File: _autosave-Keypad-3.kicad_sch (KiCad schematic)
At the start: 20 parts, among them SW1 SW_Push, U1 ATmega32U4-A, Y1 16MHz

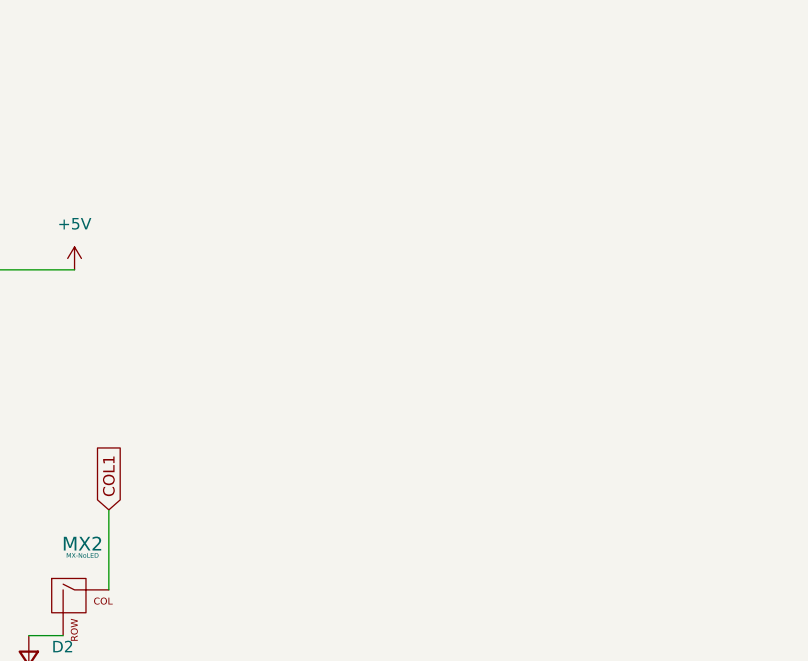
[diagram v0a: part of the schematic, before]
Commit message: Finished first board design
route is very messy, will fix soon.
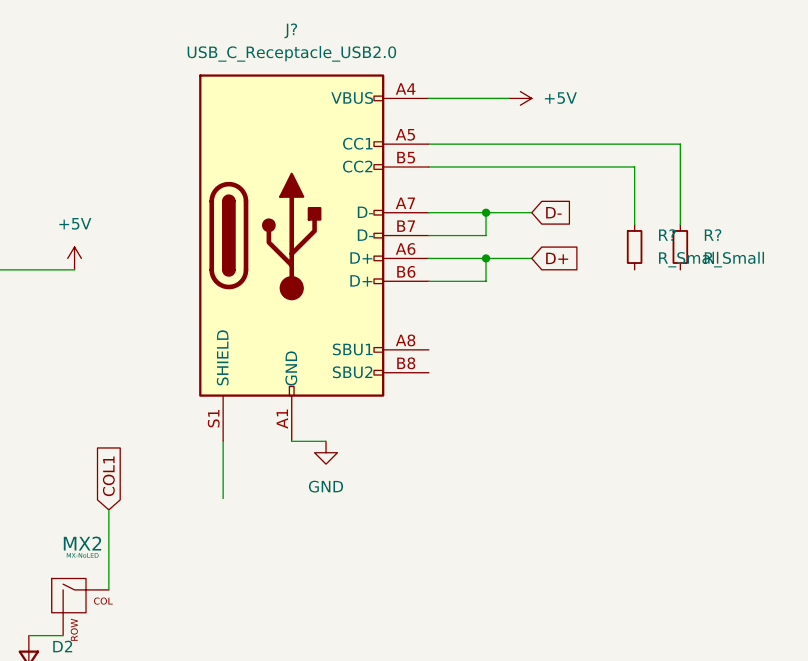
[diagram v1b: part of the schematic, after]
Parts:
- added J?: USB_C_Receptacle_USB2.0, symbol Connector:USB_C_Receptacle_USB2.0
- added R? (x2): R_Small, symbol Device:R_Small
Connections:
- net +5V: now also J?.A4 (VBUS), J?.A9 (VBUS), J?.B4 (VBUS), J?.B9 (VBUS)
- net D+: now also J?.A6 (D+), J?.B6 (D+)
- net D-: now also J?.A7 (D-), J?.B7 (D-)
- net GND: now also J?.A1 (GND), J?.A12 (GND), J?.B1 (GND), J?.B12 (GND)
- new net: J?.B5 (CC2), R?.1
- new net: J?.A5 (CC1), R?.1
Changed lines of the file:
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@@
 (kicad_sch (version 20211123) (generator eeschema)
   (paper "A4")
+  (junction (at 241.3 35.56) (diameter 0) (color 0 0 0 0)
+  )
   (junction (at 114.3 35.56) (diameter 0) (color 0 0 0 0)
   )
@@
   (junction (at 74.93 54.61) (diameter 0) (color 0 0 0 0)
   )
+  (junction (at 241.3 40.64) (diameter 0) (color 0 0 0 0)
+  )
   (junction (at 60.96 111.76) (diameter 0) (color 0 0 0 0)
   )
@@
     (stroke (width 0) (type default) (color 0 0 0 0))
   )
+  (wire (pts (xy 234.95 43.18) (xy 241.3 43.18))
+    (stroke (width 0) (type default) (color 0 0 0 0))
+  )
   (wire (pts (xy 96.52 43.18) (xy 99.06 43.18))
     (stroke (width 0) (type default) (color 0 0 0 0))
   )
+  (wire (pts (xy 212.09 60.96) (xy 212.09 67.31))
+    (stroke (width 0) (type default) (color 0 0 0 0))
+  )
   (wire (pts (xy 172.72 41.91) (xy 181.61 41.91))
     (stroke (width 0) (type default) (color 0 0 0 0))
@@
     (stroke (width 0) (type default) (color 0 0 0 0))
   )
+  (wire (pts (xy 234.95 30.48) (xy 257.81 30.48))
+    (stroke (width 0) (type default) (color 0 0 0 0))
+  )
+  (wire (pts (xy 234.95 22.86) (xy 243.84 22.86))
+    (stroke (width 0) (type default) (color 0 0 0 0))
+  )
   (wire (pts (xy 86.36 48.26) (xy 80.01 48.26))
     (stroke (width 0) (type default) (color 0 0 0 0))
@@
     (stroke (width 0) (type default) (color 0 0 0 0))
   )
+  (wire (pts (xy 234.95 35.56) (xy 241.3 35.56))
+    (stroke (width 0) (type default) (color 0 0 0 0))
+  )
+  (wire (pts (xy 257.81 30.48) (xy 257.81 36.83))
+    (stroke (width 0) (type default) (color 0 0 0 0))
+  )
   (wire (pts (xy 69.85 71.12) (xy 74.93 71.12))
     (stroke (width 0) (type default) (color 0 0 0 0))
@@
     (stroke (width 0) (type default) (color 0 0 0 0))
   )
+  (wire (pts (xy 241.3 40.64) (xy 246.38 40.64))
+    (stroke (width 0) (type default) (color 0 0 0 0))
+  )
   (wire (pts (xy 73.66 76.2) (xy 99.06 76.2))
     (stroke (width 0) (type default) (color 0 0 0 0))
   )
+  (wire (pts (xy 234.95 38.1) (xy 241.3 38.1))
+    (stroke (width 0) (type default) (color 0 0 0 0))
+  )
   (wire (pts (xy 93.98 43.18) (xy 96.52 43.18))
     (stroke (width 0) (type default) (color 0 0 0 0))
@@
     (stroke (width 0) (type default) (color 0 0 0 0))
   )
+  (wire (pts (xy 262.89 27.94) (xy 262.89 36.83))
+    (stroke (width 0) (type default) (color 0 0 0 0))
+  )
   (wire (pts (xy 83.82 50.8) (xy 83.82 55.88))
     (stroke (width 0) (type default) (color 0 0 0 0))
@@
     (stroke (width 0) (type default) (color 0 0 0 0))
   )
+  (wire (pts (xy 241.3 35.56) (xy 246.38 35.56))
+    (stroke (width 0) (type default) (color 0 0 0 0))
+  )
   (wire (pts (xy 86.36 53.34) (xy 99.06 53.34))
     (stroke (width 0) (type default) (color 0 0 0 0))
@@
     (stroke (width 0) (type default) (color 0 0 0 0))
   )
+  (wire (pts (xy 241.3 35.56) (xy 241.3 38.1))
+    (stroke (width 0) (type default) (color 0 0 0 0))
+  )
   (wire (pts (xy 66.04 106.68) (xy 76.2 106.68))
     (stroke (width 0) (type default) (color 0 0 0 0))
@@
     (stroke (width 0) (type default) (color 0 0 0 0))
   )
+  (wire (pts (xy 219.71 60.96) (xy 223.52 60.96))
+    (stroke (width 0) (type default) (color 0 0 0 0))
+  )
+  (wire (pts (xy 234.95 27.94) (xy 262.89 27.94))
+    (stroke (width 0) (type default) (color 0 0 0 0))
+  )
   (wire (pts (xy 45.72 111.76) (xy 55.88 111.76))
     (stroke (width 0) (type default) (color 0 0 0 0))
@@
     (stroke (width 0) (type default) (color 0 0 0 0))
   )
+  (wire (pts (xy 241.3 40.64) (xy 241.3 43.18))
+    (stroke (width 0) (type default) (color 0 0 0 0))
+  )
   (wire (pts (xy 55.88 111.76) (xy 60.96 111.76))
     (stroke (width 0) (type default) (color 0 0 0 0))
@@
   )
   (wire (pts (xy 74.93 54.61) (xy 74.93 58.42))
+    (stroke (width 0) (type default) (color 0 0 0 0))
+  )
+  (wire (pts (xy 234.95 40.64) (xy 241.3 40.64))
     (stroke (width 0) (type default) (color 0 0 0 0))
   )
@@
     )
   )
+  (global_label "D-" (shape input) (at 246.38 35.56 0) (fields_autoplaced)
+    (effects (font (size 1.27 1.27)) (justify left))
+    (property "Intersheet References" "${INTERSHEET_REFS}" (id 0) (at 251.6355 35.4806 0)
+      (effects (font (size 1.27 1.27)) (justify left) hide)
+    )
+  )
   (global_label "COL0" (shape input) (at 129.54 114.3 0) (fields_autoplaced)
     (effects (font (size 1.27 1.27)) (justify left))
@@
     )
   )
+  (global_label "D+" (shape input) (at 246.38 40.64 0) (fields_autoplaced)
+    (effects (font (size 1.27 1.27)) (justify left))
+    (property "Intersheet References" "${INTERSHEET_REFS}" (id 0) (at 251.6355 40.5606 0)
+      (effects (font (size 1.27 1.27)) (justify left) hide)
+    )
+  )
   (global_label "D+" (shape input) (at 69.85 68.58 180) (fields_autoplaced)
     (effects (font (size 1.27 1.27)) (justify right))
@@
     (pin "1")
     (pin "2")
+  )
+  (symbol (lib_id "power:+5V") (at 243.84 22.86 270) (unit 1)
+    (in_bom yes) (on_board yes) (fields_autoplaced)
+    (property "Reference" "#PWR?" (id 0) (at 240.03 22.86 0)
+      (effects (font (size 1.27 1.27)) hide)
+    )
+    (property "Value" "+5V" (id 1) (at 247.65 22.8599 90)
+      (effects (font (size 1.27 1.27)) (justify left))
+    )
+    (property "Footprint" "" (id 2) (at 243.84 22.86 0)
+      (effects (font (size 1.27 1.27)) hide)
+    )
+    (property "Datasheet" "" (id 3) (at 243.84 22.86 0)
+      (effects (font (size 1.27 1.27)) hide)
+    )
+    (pin "1")
   )
   (symbol (lib_id "power:+5V") (at 195.58 41.91 0) (unit 1)
@@
     (pin "2")
   )
+  (symbol (lib_id "Device:R_Small") (at 257.81 39.37 0) (unit 1)
+    (in_bom yes) (on_board yes) (fields_autoplaced)
+    (property "Reference" "R?" (id 0) (at 260.35 38.0999 0)
+      (effects (font (size 1.27 1.27)) (justify left))
+    )
+    (property "Value" "R_Small" (id 1) (at 260.35 40.6399 0)
+      (effects (font (size 1.27 1.27)) (justify left))
+    )
+    (property "Footprint" "" (id 2) (at 257.81 39.37 0)
+      (effects (font (size 1.27 1.27)) hide)
+    )
+    (property "Datasheet" "~" (id 3) (at 257.81 39.37 0)
+      (effects (font (size 1.27 1.27)) hide)
+    )
+    (pin "1")
+    (pin "2")
+  )
   (symbol (lib_id "power:GND") (at 73.66 85.09 0) (unit 1)
     (in_bom yes) (on_board yes) (fields_autoplaced)
@@
     (pin "2")
   )
+  (symbol (lib_id "Device:R_Small") (at 262.89 39.37 0) (unit 1)
+    (in_bom yes) (on_board yes) (fields_autoplaced)
+    (property "Reference" "R?" (id 0) (at 265.43 38.0999 0)
+      (effects (font (size 1.27 1.27)) (justify left))
+    )
+    (property "Value" "R_Small" (id 1) (at 265.43 40.6399 0)
+      (effects (font (size 1.27 1.27)) (justify left))
+    )
+    (property "Footprint" "" (id 2) (at 262.89 39.37 0)
+      (effects (font (size 1.27 1.27)) hide)
+    )
+    (property "Datasheet" "~" (id 3) (at 262.89 39.37 0)
+      (effects (font (size 1.27 1.27)) hide)
+    )
+    (pin "1")
+    (pin "2")
+  )
   (symbol (lib_id "Device:C_Small") (at 66.04 109.22 0) (unit 1)
     (in_bom yes) (on_board yes) (fields_autoplaced)
@@
     )
     (pin "1")
+  )
+  (symbol (lib_id "Connector:USB_C_Receptacle_USB2.0") (at 219.71 38.1 0) (unit 1)
+    (in_bom yes) (on_board yes) (fields_autoplaced)
+    (property "Reference" "J?" (id 0) (at 219.71 15.24 0))
+    (property "Value" "USB_C_Receptacle_USB2.0" (id 1) (at 219.71 17.78 0))
+    (property "Footprint" "" (id 2) (at 223.52 38.1 0)
+      (effects (font (size 1.27 1.27)) hide)
+    )
+    (property "Datasheet" "https://www.usb.org/sites/default/files/documents/usb_type-c.zip" (id 3) (at 223.52 38.1 0)
+      (effects (font (size 1.27 1.27)) hide)
+    )
+    (pin "A1")
+    (pin "A12")
+    (pin "A4")
+    (pin "A5")
+    (pin "A6")
+    (pin "A7")
+    (pin "A8")
+    (pin "A9")
+    (pin "B1")
+    (pin "B12")
+    (pin "B4")
+    (pin "B5")
+    (pin "B6")
+    (pin "B7")
+    (pin "B8")
+    (pin "B9")
+    (pin "S1")
   )
   (symbol (lib_id "Device:Crystal_GND24_Small") (at 86.36 50.8 270) (unit 1)
@@
     (pin "1")
   )
+  (symbol (lib_id "power:GND") (at 223.52 60.96 0) (unit 1)
+    (in_bom yes) (on_board yes) (fields_autoplaced)
+    (property "Reference" "#PWR?" (id 0) (at 223.52 67.31 0)
+      (effects (font (size 1.27 1.27)) hide)
+    )
+    (property "Value" "GND" (id 1) (at 223.52 66.04 0))
+    (property "Footprint" "" (id 2) (at 223.52 60.96 0)
+      (effects (font (size 1.27 1.27)) hide)
+    )
+    (property "Datasheet" "" (id 3) (at 223.52 60.96 0)
+      (effects (font (size 1.27 1.27)) hide)
+    )
+    (pin "1")
+  )
   (sheet_instances
     (path "/" (page "1"))
@@
       (reference "#PWR0113") (unit 1) (value "VCC") (footprint "")
     )
+    (path "/3c27b9f9-2ba8-4150-8cd7-fc6b702be7b9"
+      (reference "#PWR?") (unit 1) (value "+5V") (footprint "")
+    )
+    (path "/ff0f6824-7994-4850-9e6c-74e9b0f18f76"
+      (reference "#PWR?") (unit 1) (value "GND") (footprint "")
+    )
     (path "/ad0e28b6-1443-4065-afe7-dc2a56df346b"
       (reference "C1") (unit 1) (value "22pf") (footprint "Capacitor_SMD:C_0805_2012Metric")
@@
       (reference "F1") (unit 1) (value "500mA") (footprint "Fuse:Fuse_1206_3216Metric")
     )
+    (path "/dcf57bfd-08d4-4b5b-9245-8eb742026298"
+      (reference "J?") (unit 1) (value "USB_C_Receptacle_USB2.0") (footprint "")
+    )
     (path "/728e0df7-77d3-4862-b864-13cb45a6d3ad"
       (reference "MX1") (unit 1) (value "MX-NoLED") (footprint "MX_Alps_Hybrid:MX-1U-NoLED")
@@
       (reference "R4") (unit 1) (value "10k") (footprint "Resistor_SMD:R_0805_2012Metric")
     )
+    (path "/92bf1bda-7ed4-400d-a9ba-1bd9be26b386"
+      (reference "R?") (unit 1) (value "R_Small") (footprint "")
+    )
+    (path "/bff8d1ee-2e66-44a7-b201-78e488a94293"
+      (reference "R?") (unit 1) (value "R_Small") (footprint "")
+    )
     (path "/2cf5b7a3-2d48-4fa1-8fbe-792d77e7e3d8"
